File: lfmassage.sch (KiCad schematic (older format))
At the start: 26 parts, among them J1 Batt, J2 OUT, J3 ESP_DEVKITC, Q1 BFS20W, SW1 NW3-A03-05, SW2 SW_Push, SW3 SW_Push, SW4 SW_Push, U1 USB_CType_6Pin, U2 MCP73831

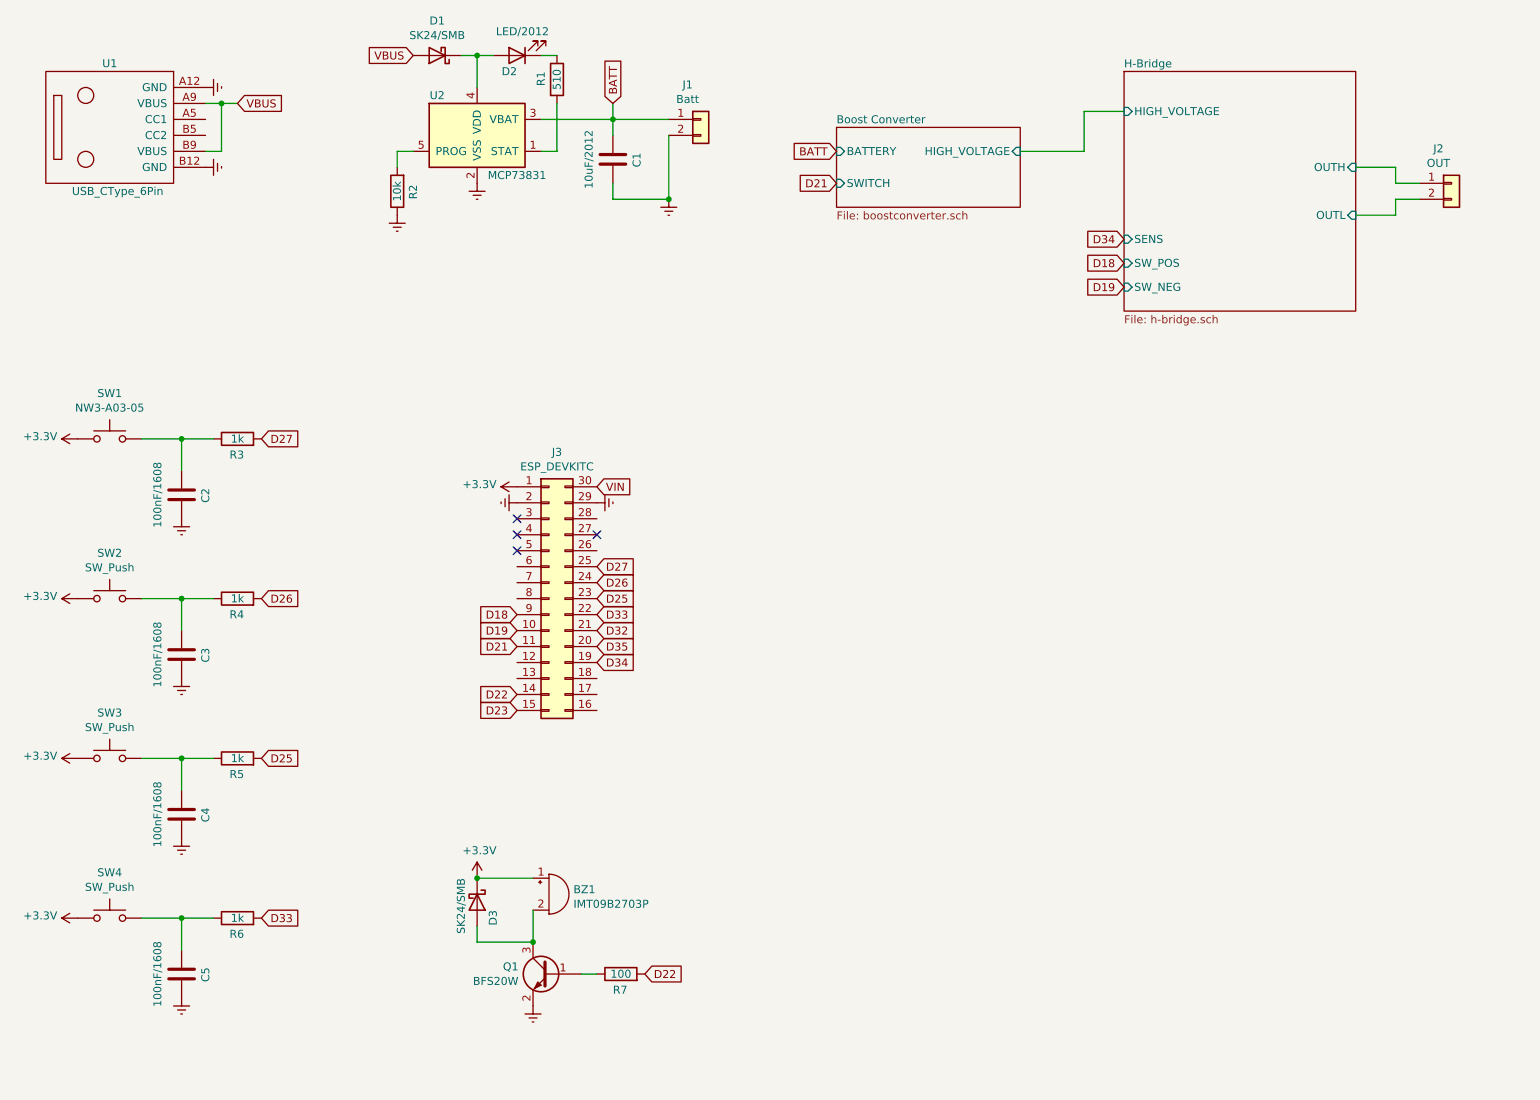
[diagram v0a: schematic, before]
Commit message: 2021-09-06
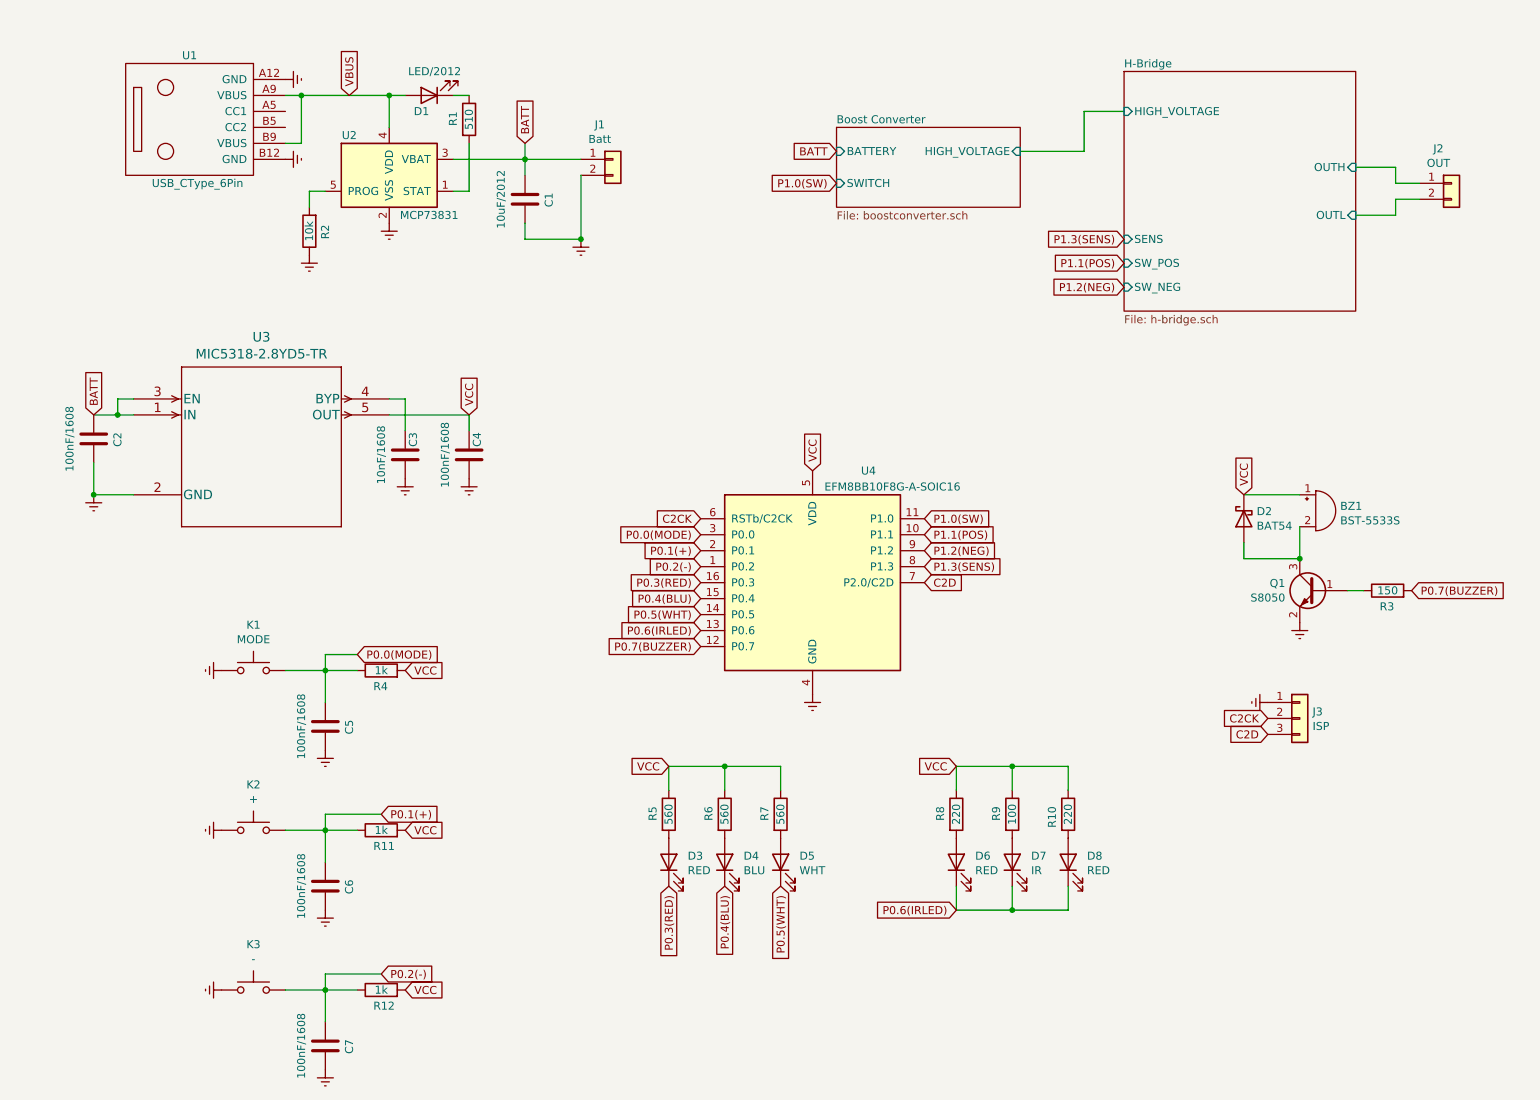
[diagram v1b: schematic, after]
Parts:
- removed C5: 100nF/1608, Capacitor_SMD:C_0603_1608Metric_Pad1.08x0.95mm_HandSolder, symbol Device:C
- removed D1, D3: SK24/SMB, Diode_SMD:D_SMB_Handsoldering, symbol Device:D_Schottky
- removed J3: ESP_DEVKITC, espressif:ESP32_DEVKITC, symbol Connector_Generic:Conn_02x15_Counter_Clockwise
- removed SW2, SW3, SW4: SW_Push, ali_Switch:NW3-A03-05, symbol Switch:SW_Push
- added C2, C4: 100nF/1608, Capacitor_SMD:C_0603_1608Metric_Pad1.08x0.95mm_HandSolder, symbol Device:C
- added C3: 10nF/1608, Capacitor_SMD:C_0603_1608Metric_Pad1.08x0.95mm_HandSolder, symbol Device:C
- added D2: BAT54, Diode_SMD:D_SOT-23_ANK, symbol Diode:BAT54J
- added D3: RED, LED_SMD:LED_0603_1608Metric, symbol Device:LED
- added D4: BLU, LED_SMD:LED_0603_1608Metric, symbol Device:LED
- added D5: WHT, LED_SMD:LED_0603_1608Metric, symbol Device:LED
- added D6, D8: RED, LED_SMD:LED_1206_3216Metric, symbol Device:LED
- added D7: IR, LED_SMD:LED_1206_3216Metric, symbol Device:LED
- added J3: ISP, Connector_PinHeader_2.54mm:PinHeader_1x03_P2.54mm_Vertical, symbol Connector_Generic:Conn_01x03
- added K2: +, Button_Switch_SMD:SW_SPST_B3SL-1002P, symbol Switch:SW_Push
- added K3: -, Button_Switch_SMD:SW_SPST_B3SL-1002P, symbol Switch:SW_Push
- added R10, R8: 220, Resistor_SMD:R_0603_1608Metric_Pad0.98x0.95mm_HandSolder, symbol Device:R
- added R5, R7: 560, Resistor_SMD:R_0603_1608Metric_Pad0.98x0.95mm_HandSolder, symbol Device:R
- added R9: 100, Resistor_SMD:R_0603_1608Metric_Pad0.98x0.95mm_HandSolder, symbol Device:R
- added U3: MIC5318-2.8YD5-TR, Package_TO_SOT_SMD:TSOT-23-5, symbol MIC531833YD5TR:MIC5318-3.3YD5-TR
- added U4: EFM8BB10F8G-A-SOIC16, Package_SO:SOIC-16_3.9x9.9mm_P1.27mm, symbol MCU_SiliconLabs:EFM8BB10F8G-A-SOIC16
- BZ1: value IMT09B2703P -> BST-5533S; footprint Buzzer_Beeper:MagneticBuzzer_PUI_AT-0927-TT-6-R -> buzzer:BST-5533S; MPN (none) -> BST-5533S
- K1: renamed from SW1; value NW3-A03-05 -> MODE; footprint ali_Switch:NW3-A03-05 -> Button_Switch_SMD:SW_SPST_B3SL-1002P; MPN (none) -> PTS526
- Q1: value BFS20W -> S8050
- R3: renamed from R7; value 100 -> 150
- R6: value 1k -> 560
- renumbered C2 to C5, C3 to C6, C4 to C7, D2 to D1, R4 to R11, R5 to R12, R3 to R4
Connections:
- net D25 is gone; now on net VCC: R12.2
- net D26 is gone; now on net VCC: R11.2
- net D27 is gone; now on net VCC: R4.2
- net BATT: now also C2.1, U3.1 (IN), U3.3 (EN)
- net Earth: now also K1.1, C2.2, C3.2, C4.2, J3.1 (Pin_1), K2.1, K3.1, U3.2 (GND), U4.4 (GND)
- net VBUS: now also D1.2 (A), U2.4 (VDD)
- net P0.0(MODE): now reaches C5.1, K1.2, R4.1
- net P0.0(MODE): now also U4.3 (P0.0)
- net P0.1(+): now reaches C6.1, R11.1
- net P0.1(+): now also K2.2, U4.2 (P0.1)
- net P0.2(-): now reaches C7.1, R12.1
- net P0.2(-): now also K3.2, U4.1 (P0.2)
- net VCC: now reaches R6.1
- net VCC: now also BZ1.1 (-), C4.1, D2.1 (K), R10.1, R5.1, R7.1, R8.1, R9.1, U3.5 (OUT), U4.5 (VDD)
- net at BZ1.2 (+), Q1.3 (C): now also D2.2 (A)
- removed net +3V3: BZ1.1 (-), K1.1
- net D22 renamed P0.7(BUZZER)
- net P0.7(BUZZER): now also U4.12 (P0.7)
- net D33: no longer names the net of R6.2
- net D33: now also D4.2 (A)
- new net: C3.1, U3.4 (BYP)
- new net: D6.2 (A), R8.2
- new net: D7.2 (A), R9.2
- new net: D8.2 (A), R10.2
- new net: D3.2 (A), R5.2
- new net: D5.2 (A), R7.2
- new net C2CK: J3.2 (Pin_2), U4.6 (RSTb/C2CK)
- new net C2D: J3.3 (Pin_3), U4.7 (P2.0/C2D)
- new net P0.3(RED): D3.1 (K), U4.16 (P0.3)
- new net P0.4(BLU): D4.1 (K), U4.15 (P0.4)
- new net P0.5(WHT): D5.1 (K), U4.14 (P0.5)
- new net P0.6(IRLED): D6.1 (K), D7.1 (K), D8.1 (K), U4.13 (P0.6)
- new net P1.0(SW): U4.11 (P1.0)
- new net P1.1(POS): U4.10 (P1.1)
- new net P1.2(NEG): U4.9 (P1.2)
- new net P1.3(SENS): U4.8 (P1.3)
- no-connect marks 4 -> 0
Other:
- moved on the sheet: BZ1, C1, C5, C6, C7, D1, J1, K1, Q1, R1, R11, R12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
